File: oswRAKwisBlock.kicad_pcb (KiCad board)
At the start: 2 copper layers, 33.8 x 46 mm, 8 parts, among them J1 WisBlock, J2 0524352471

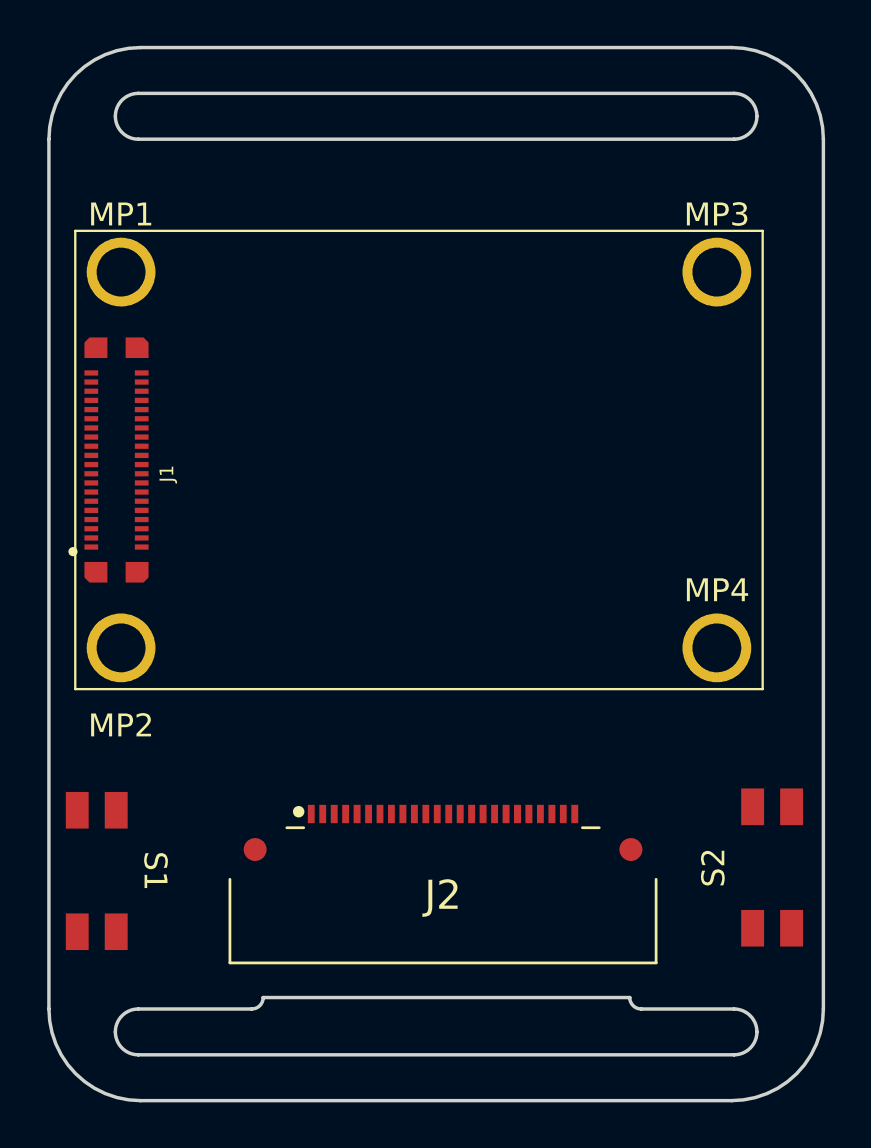
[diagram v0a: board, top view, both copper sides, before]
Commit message: Updates.
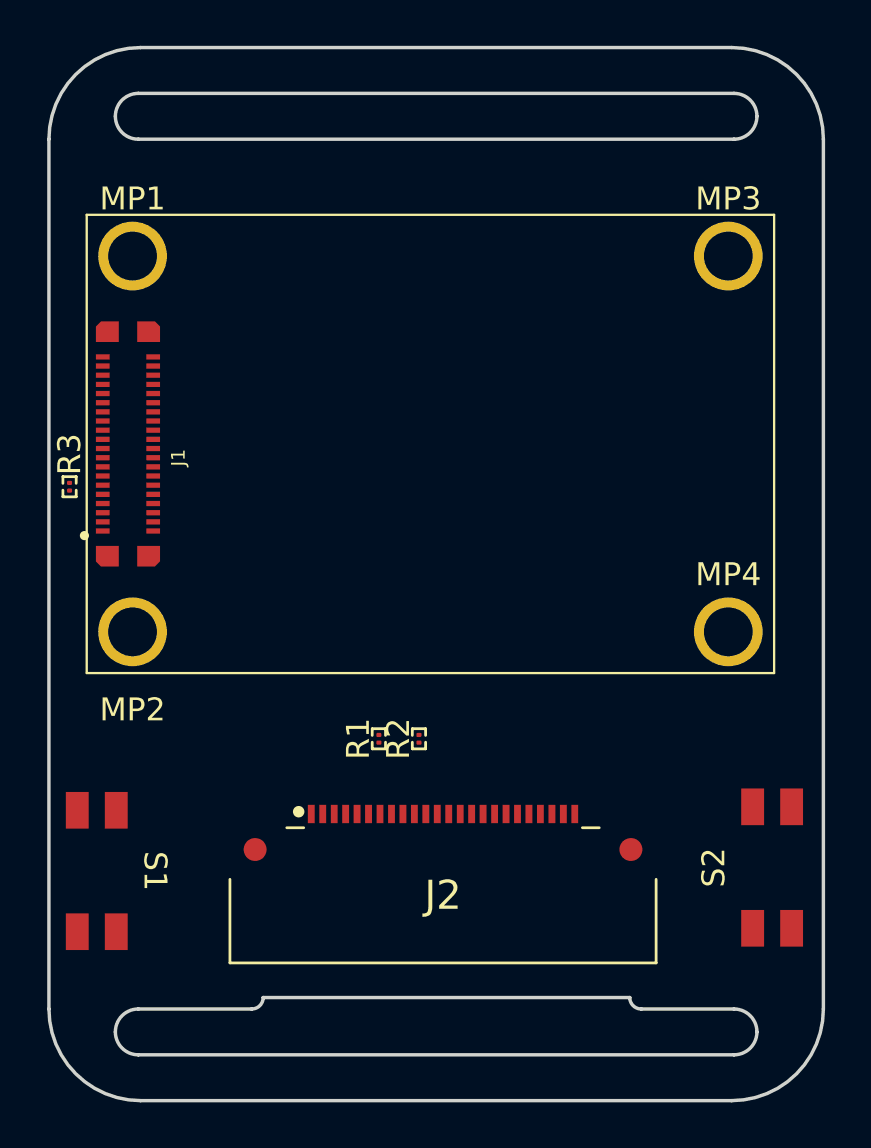
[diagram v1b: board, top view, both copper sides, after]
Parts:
- added R1: 10k, AllardChip:RESC40X20X15L10N, F.Cu at (134.2, 130.2)
- added R2: 10k, AllardChip:RESC40X20X15L10N, F.Cu at (136.0, 130.2)
- added R3: 10k, AllardChip:RESC40X20X15L10N, F.Cu at (120.8, 119.2)
- moved J1 0.86 mm to (123.3, 117.3)
- moved MP1 0.86 mm to (123.5, 109.1)
- moved MP2 0.86 mm to (123.5, 125.5)
- moved MP3 0.86 mm to (149.5, 109.1)
- moved MP4 0.86 mm to (149.5, 125.5)
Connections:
- J1 pad 13: unconnected-(J1-RESET-Pad13) -> Net-(J1-RESET)
- J1 pad 39: unconnected-(J1-FS3-Pad39) -> GND
- J1 pad 40: unconnected-(J1-GND-Pad40) -> GND
- J1 pad 5: unconnected-(J1-3V3-Pad5) -> VDD
- J1 pad FS1: unconnected-(J1-GND-PadFS1) -> GND
- J1 pad FS2: unconnected-(J1-GND-PadFS2) -> GND
- J1 pad FS4: unconnected-(J1-GND-PadFS4) -> GND
- S1 pad 1: unconnected-(S1-Pad1) -> Net-(R1-Pad2)
- S1 pad 2: unconnected-(S1-Pad2) -> Net-(R1-Pad2)
- S1 pad 3: unconnected-(S1-K-Pad3) -> GND
- S1 pad 4: unconnected-(S1-A-Pad4) -> GND
- S2 pad 1: unconnected-(S2-Pad1) -> Net-(R2-Pad2)
- S2 pad 2: unconnected-(S2-Pad2) -> Net-(R2-Pad2)
- S2 pad 3: unconnected-(S2-K-Pad3) -> GND
- S2 pad 4: unconnected-(S2-A-Pad4) -> GND

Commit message: Working forward.
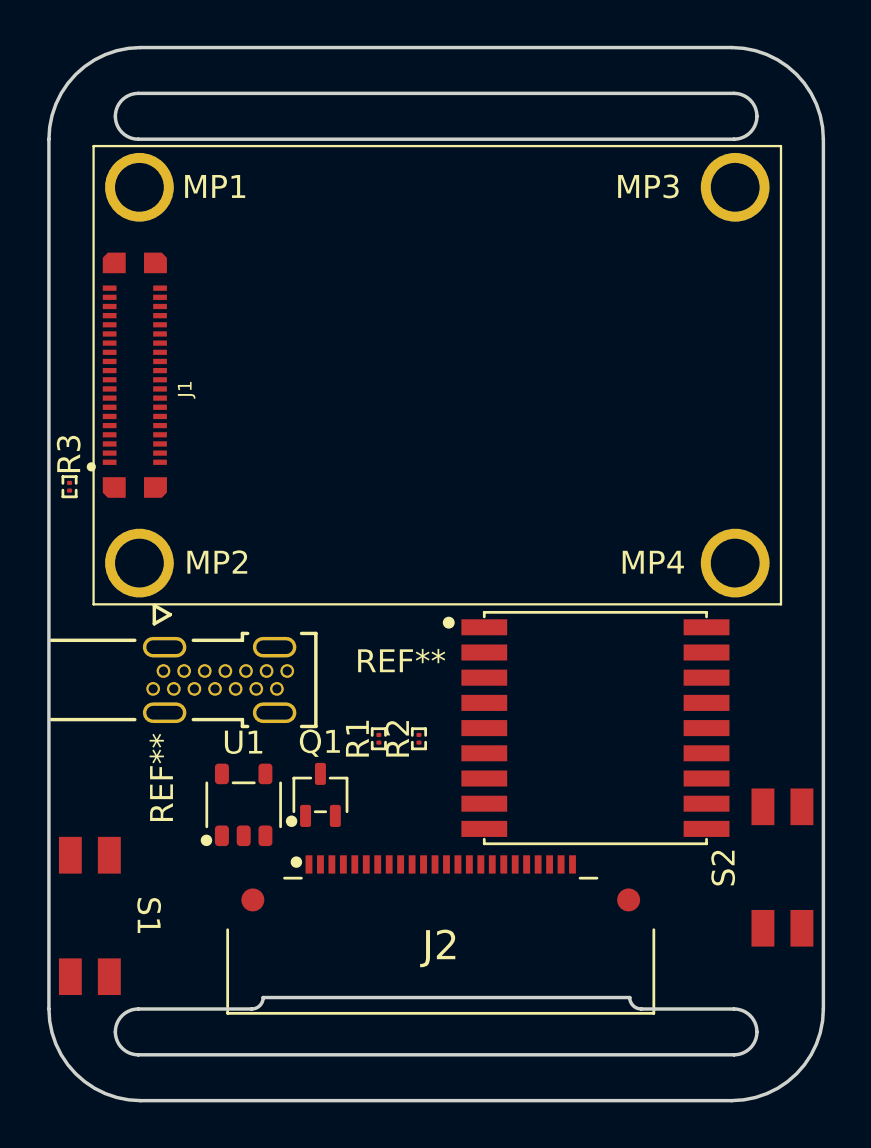
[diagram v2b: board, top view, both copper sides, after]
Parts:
- added Q1: SI1308EDL-T1-GE3, AllardSOT:SOT23-3P65_210X110L20X32N, F.Cu at (131.7, 132.6)
- added REF**: SIMCOM_SIM68M, AllardSpecialFootPrints:SIMCOM_SIM68M, F.Cu at (143.7, 129.7)
- added REF**: MOLEX_2169890001, AllardConnFootPrints:MOLEX_2169890001, F.Cu at (119.8, 127.6)
- added U1: MCP73811T-420I/OT, AllardSOT:SOT23-5P95_270X145L35X35N, F.Cu at (128.3, 133.1)
- moved MP3 3.01 mm to (149.8, 106.1)
- moved MP4 3.01 mm to (149.8, 122.5)
- moved J1 3.01 mm to (123.6, 114.3)
- moved MP1 3.01 mm to (123.8, 106.1)
- moved MP2 3.01 mm to (123.8, 122.5)
- moved J2 2.20 mm to (136.9, 139.2)
- moved S1 1.99 mm to (121.6, 137.9)
- moved S2 0.45 mm to (151.9, 135.8)
